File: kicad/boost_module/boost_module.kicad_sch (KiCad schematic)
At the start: 35 parts, among them J1 Conn_01x02, J2 Conn_01x02, J3 Conn_01x02, U1 OPA1612AxD

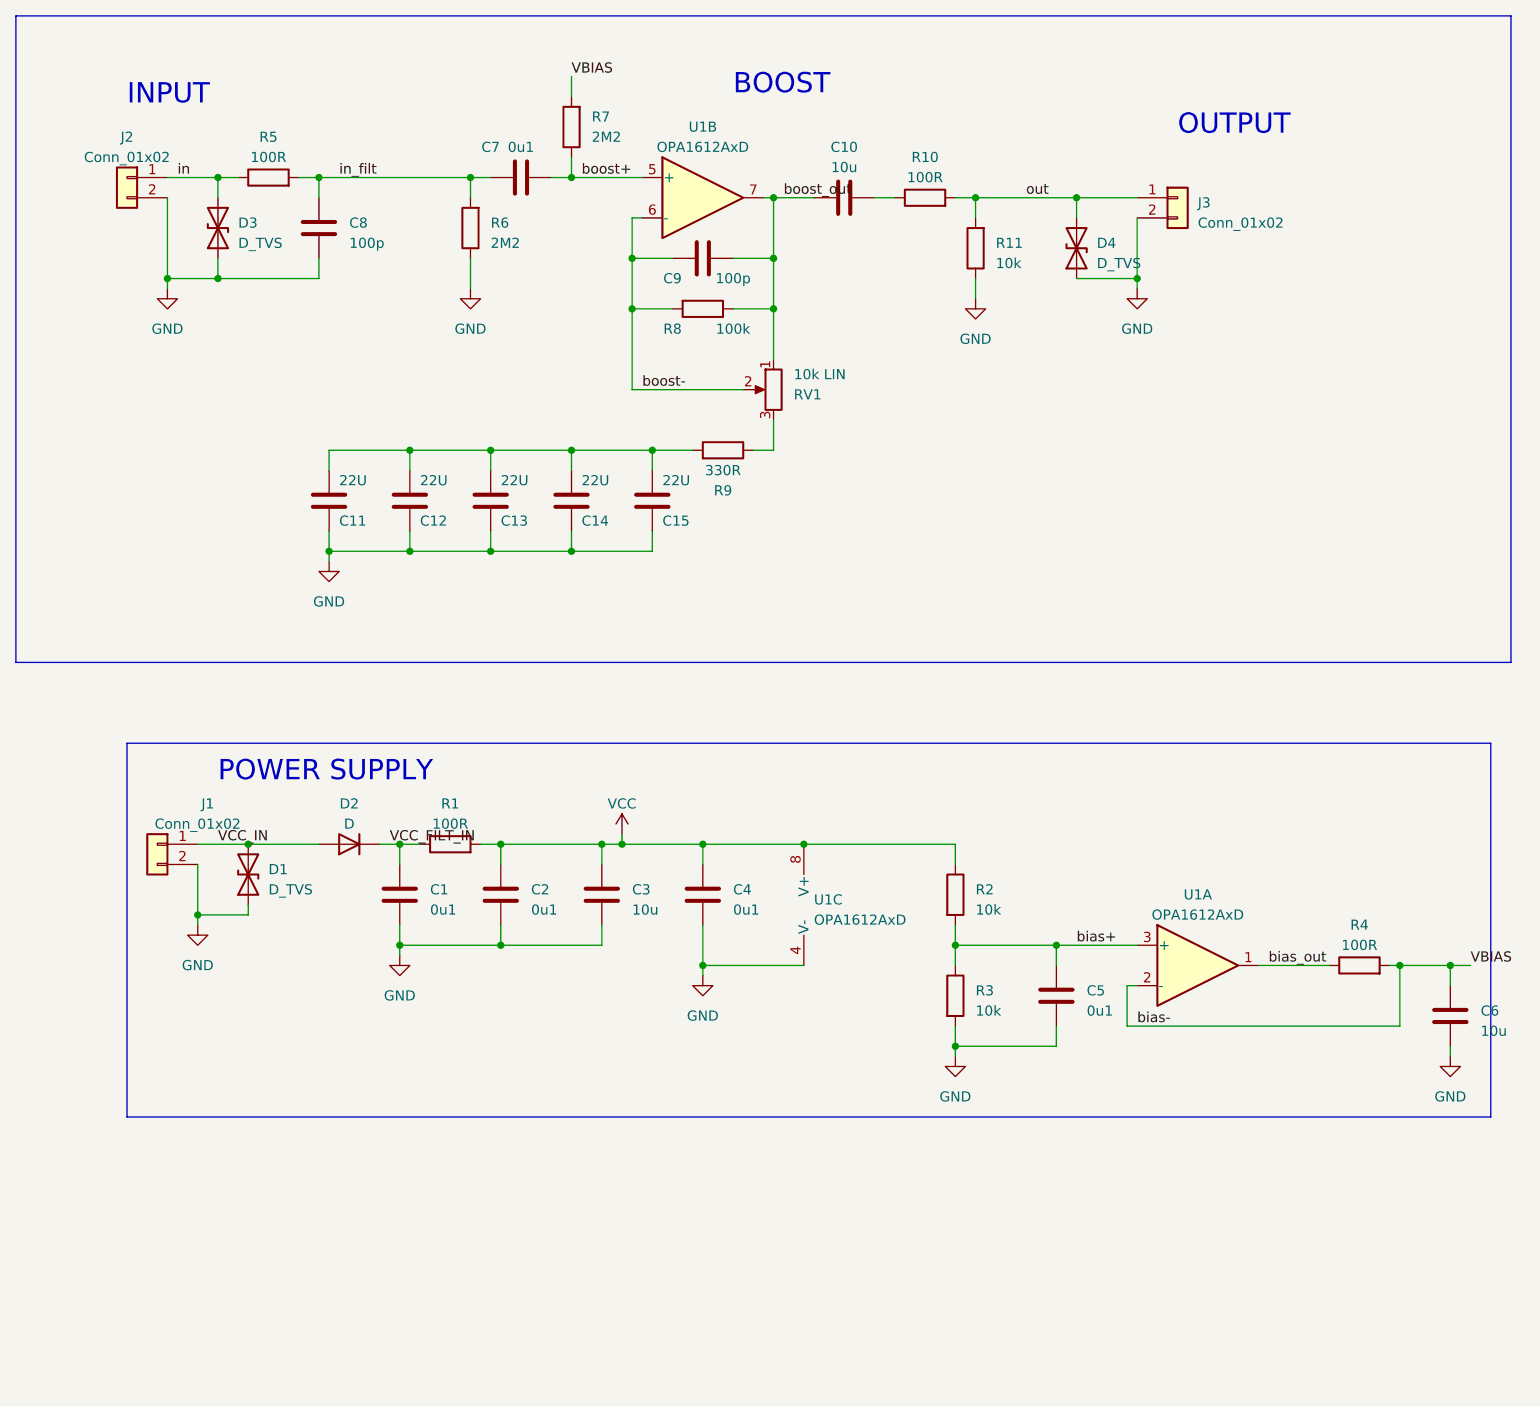
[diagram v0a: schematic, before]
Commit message: initial placement
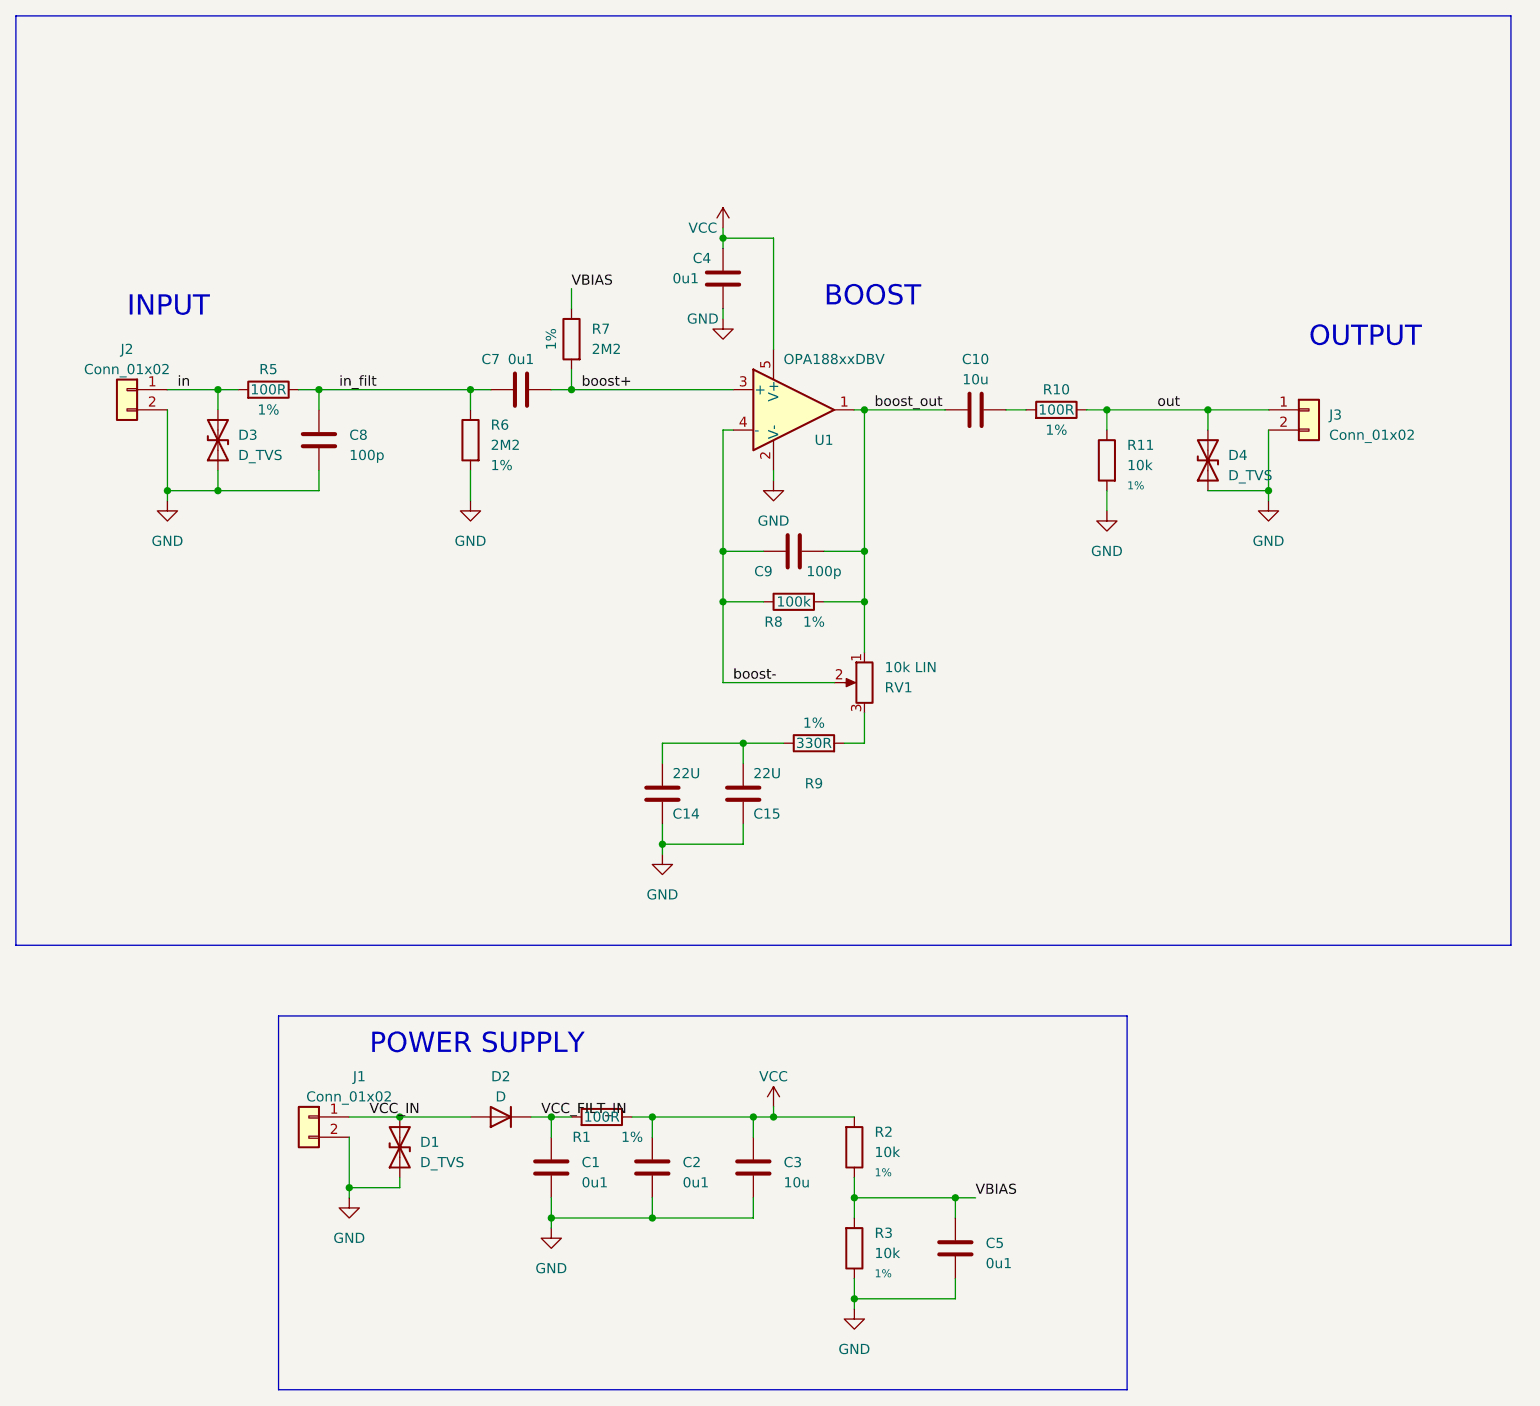
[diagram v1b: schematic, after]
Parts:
- removed C11, C12, C13: 22U, Capacitor_SMD:C_1210_3225Metric_Pad1.33x2.70mm_HandSolder, symbol Device:C
- removed C6: 10u, Capacitor_SMD:C_0603_1608Metric_Pad1.08x0.95mm_HandSolder, symbol Device:C
- removed R4: 100R, Resistor_SMD:R_0603_1608Metric_Pad0.98x0.95mm_HandSolder, symbol Device:R
- removed U1: OPA1612AxD, Package_SO:SOIC-8_3.9x4.9mm_P1.27mm, symbol Amplifier_Operational:OPA1612AxD
- added U1: OPA188xxDBV, Package_TO_SOT_SMD:TSOT-23-5, symbol Amplifier_Operational:OPA188xxDBV
- R1, R10, R5: footprint Resistor_SMD:R_0603_1608Metric_Pad0.98x0.95mm_HandSolder -> resistors:R_0603_1608Metric; symbol Device:R -> resistors:R-100R-1%-0603; MPN1 (none) -> RC0603FR-07100RL; Power (none) -> 1/10W; Tolerance (none) -> 1%
- R11, R2, R3: footprint Resistor_SMD:R_0603_1608Metric_Pad0.98x0.95mm_HandSolder -> resistors:R_0603_1608Metric; symbol Device:R -> resistors:R-10k-1%-0603; MPN1 (none) -> RC0603FR-0710KL; Power (none) -> 1/10W; Tolerance (none) -> 1%
- R6, R7: footprint Resistor_SMD:R_0603_1608Metric_Pad0.98x0.95mm_HandSolder -> resistors:R_0603_1608Metric; symbol Device:R -> resistors:R-2M2-1%-0603; MPN1 (none) -> RC0603FR-072M2L; Power (none) -> 1/10W; Tolerance (none) -> 1%
- R8: footprint Resistor_SMD:R_0603_1608Metric_Pad0.98x0.95mm_HandSolder -> resistors:R_0603_1608Metric; symbol Device:R -> resistors:R-100k-1%-0603; MPN1 (none) -> RC0603FR-07100KL; Power (none) -> 1/10W; Tolerance (none) -> 1%
- R9: footprint Resistor_SMD:R_0603_1608Metric_Pad0.98x0.95mm_HandSolder -> resistors:R_0603_1608Metric; symbol Device:R -> resistors:R-330R-1%-0603; MPN1 (none) -> RC0603FR-07330RL; Power (none) -> 1/10W; Tolerance (none) -> 1%
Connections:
- net bias+ is gone; now on net VBIAS: C5.1, R2.2, R3.1
- net GND: now also U1.2 (V-)
- net VCC: now also U1.5 (V+)
- net boost+: now also U1.3 (+)
- net boost-: now also U1.4 (-)
- net boost_out: now also U1.1
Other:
- moved on the sheet: C1, C10, C14, C15, C2, C3, C4, C5, C7, C8, C9, D1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
